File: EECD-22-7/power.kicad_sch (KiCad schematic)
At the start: 28 parts, among them Q1 IRF6616, Q2 IRF6616, U3 LMR54406DBVR, U4 LMR54406DBVR, U5 LMR54406DBVR

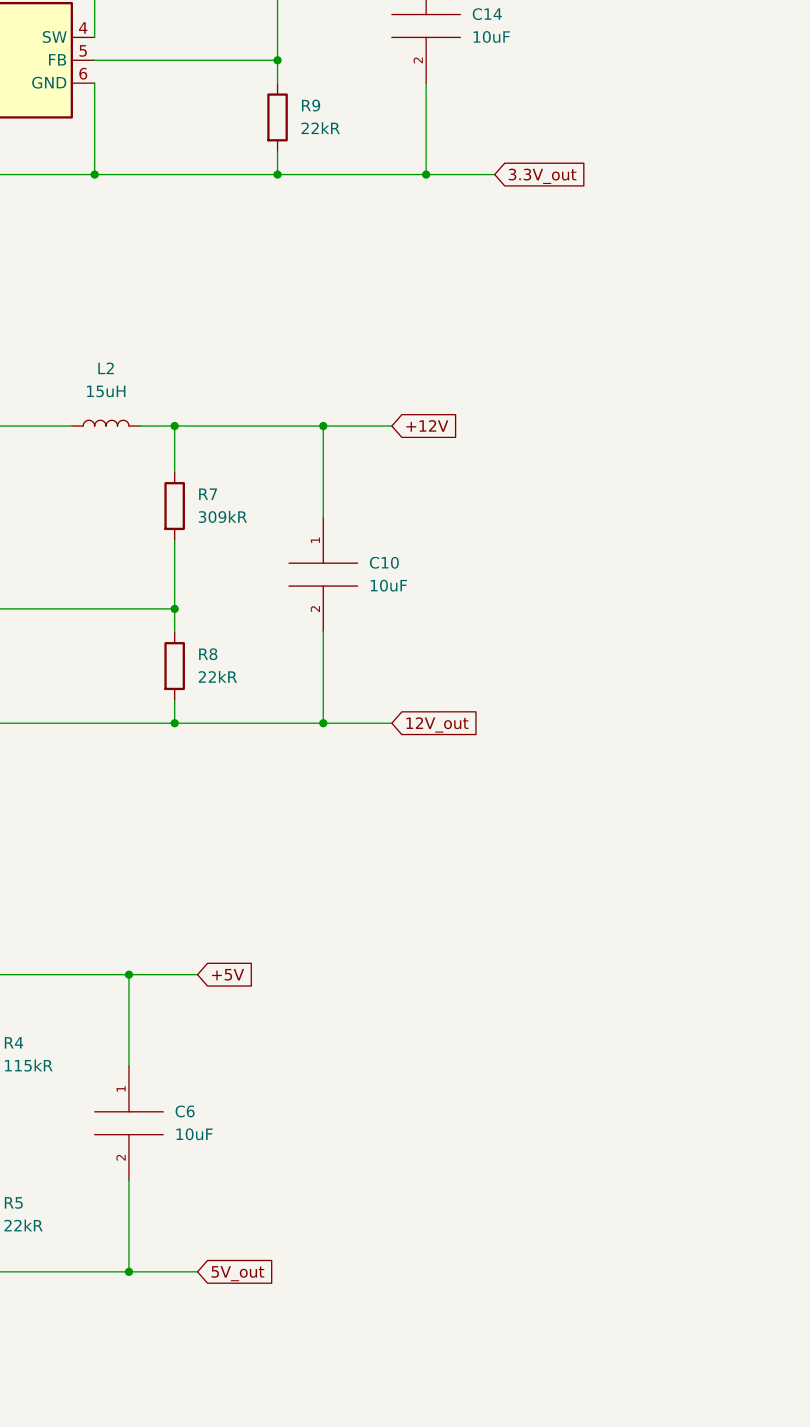
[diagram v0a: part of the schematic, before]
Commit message: Add files via upload
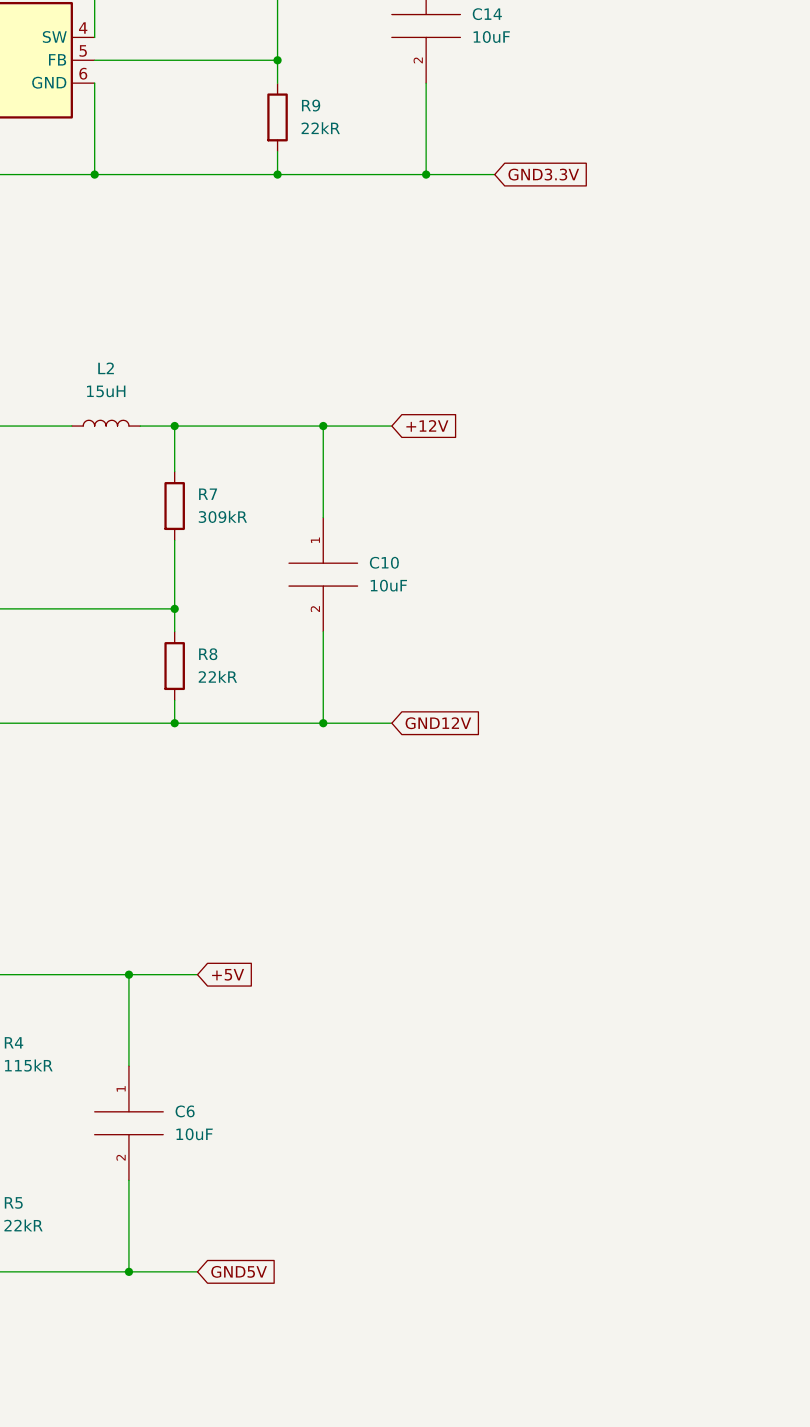
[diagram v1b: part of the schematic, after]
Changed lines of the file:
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@@
     )
   )
-  (global_label "12V_out" (shape input) (at 173.99 119.38 0) (fields_autoplaced)
+  (global_label "GND12V" (shape input) (at 173.99 119.38 0) (fields_autoplaced)
     (effects (font (size 1.27 1.27)) (justify left))
-    (property "Intersheet References" "${INTERSHEET_REFS}" (id 0) (at 183.9021 119.3006 0)
+    (property "Intersheet References" "${INTERSHEET_REFS}" (id 0) (at 183.7812 119.3006 0)
       (effects (font (size 1.27 1.27)) (justify left) hide)
     )
   )
-  (global_label "5V_out" (shape input) (at 152.4 180.34 0) (fields_autoplaced)
+  (global_label "GND5V" (shape input) (at 152.4 180.34 0) (fields_autoplaced)
     (effects (font (size 1.27 1.27)) (justify left))
-    (property "Intersheet References" "${INTERSHEET_REFS}" (id 0) (at 161.1026 180.2606 0)
+    (property "Intersheet References" "${INTERSHEET_REFS}" (id 0) (at 160.9817 180.2606 0)
       (effects (font (size 1.27 1.27)) (justify left) hide)
     )
@@
     )
   )
-  (global_label "3.3V_out" (shape input) (at 185.42 58.42 0) (fields_autoplaced)
+  (global_label "GND3.3V" (shape input) (at 185.42 58.42 0) (fields_autoplaced)
     (effects (font (size 1.27 1.27)) (justify left))
-    (property "Intersheet References" "${INTERSHEET_REFS}" (id 0) (at 195.9369 58.3406 0)
+    (property "Intersheet References" "${INTERSHEET_REFS}" (id 0) (at 195.816 58.3406 0)
       (effects (font (size 1.27 1.27)) (justify left) hide)
     )

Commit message: Add files via upload
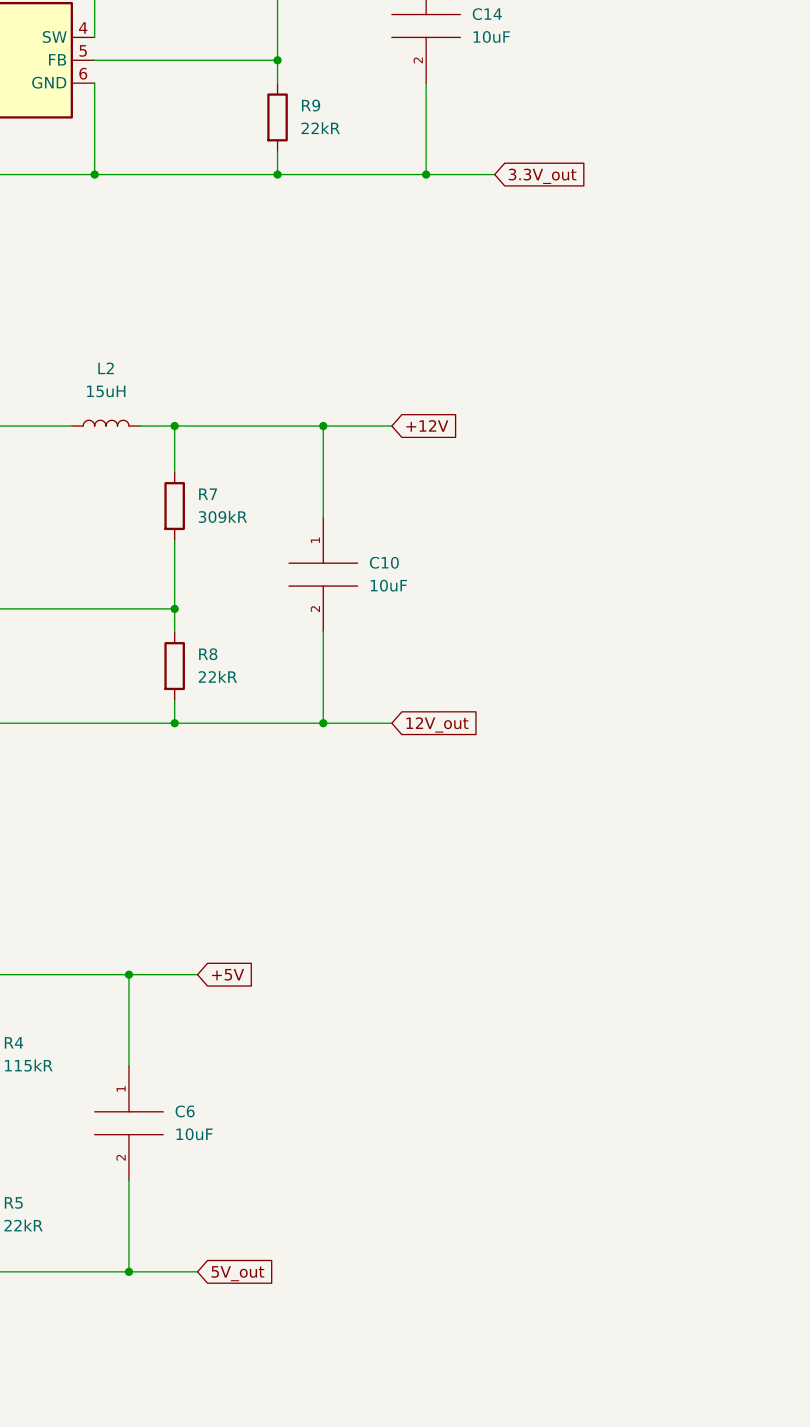
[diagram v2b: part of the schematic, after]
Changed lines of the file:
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@@
     )
   )
-  (global_label "GND12V" (shape input) (at 173.99 119.38 0) (fields_autoplaced)
+  (global_label "12V_out" (shape input) (at 173.99 119.38 0) (fields_autoplaced)
     (effects (font (size 1.27 1.27)) (justify left))
-    (property "Intersheet References" "${INTERSHEET_REFS}" (id 0) (at 183.7812 119.3006 0)
+    (property "Intersheet References" "${INTERSHEET_REFS}" (id 0) (at 183.9021 119.3006 0)
       (effects (font (size 1.27 1.27)) (justify left) hide)
     )
   )
-  (global_label "GND5V" (shape input) (at 152.4 180.34 0) (fields_autoplaced)
+  (global_label "5V_out" (shape input) (at 152.4 180.34 0) (fields_autoplaced)
     (effects (font (size 1.27 1.27)) (justify left))
-    (property "Intersheet References" "${INTERSHEET_REFS}" (id 0) (at 160.9817 180.2606 0)
+    (property "Intersheet References" "${INTERSHEET_REFS}" (id 0) (at 161.1026 180.2606 0)
       (effects (font (size 1.27 1.27)) (justify left) hide)
     )
@@
     )
   )
-  (global_label "GND3.3V" (shape input) (at 185.42 58.42 0) (fields_autoplaced)
+  (global_label "3.3V_out" (shape input) (at 185.42 58.42 0) (fields_autoplaced)
     (effects (font (size 1.27 1.27)) (justify left))
-    (property "Intersheet References" "${INTERSHEET_REFS}" (id 0) (at 195.816 58.3406 0)
+    (property "Intersheet References" "${INTERSHEET_REFS}" (id 0) (at 195.9369 58.3406 0)
       (effects (font (size 1.27 1.27)) (justify left) hide)
     )
